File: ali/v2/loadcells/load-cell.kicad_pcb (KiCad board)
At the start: 4 copper layers, 85 x 76 mm, 108 parts, among them J1 Conn_02x01, J10 Conn_01x04, J11 Conn_01x04, J12 Conn_01x04, J2 Conn_01x05, J26 Vertical Ethernet, J3 USB_C_Receptacle_USB2.0_16P, J4 Conn_01x15, J5 Conn_02x09_Counter_Clockwise, J6 Screw_Terminal_01x02, J8 Conn_01x03, J9 Conn_01x04, SW1 SKRPANE010, U1 STM32H563RIV6, U2 AP2112K-3.3, U4 TJA1462ATK, U6 ADS124S08, U7 LAN8742AI, Y1 25 MHz, Y2 25 MHz

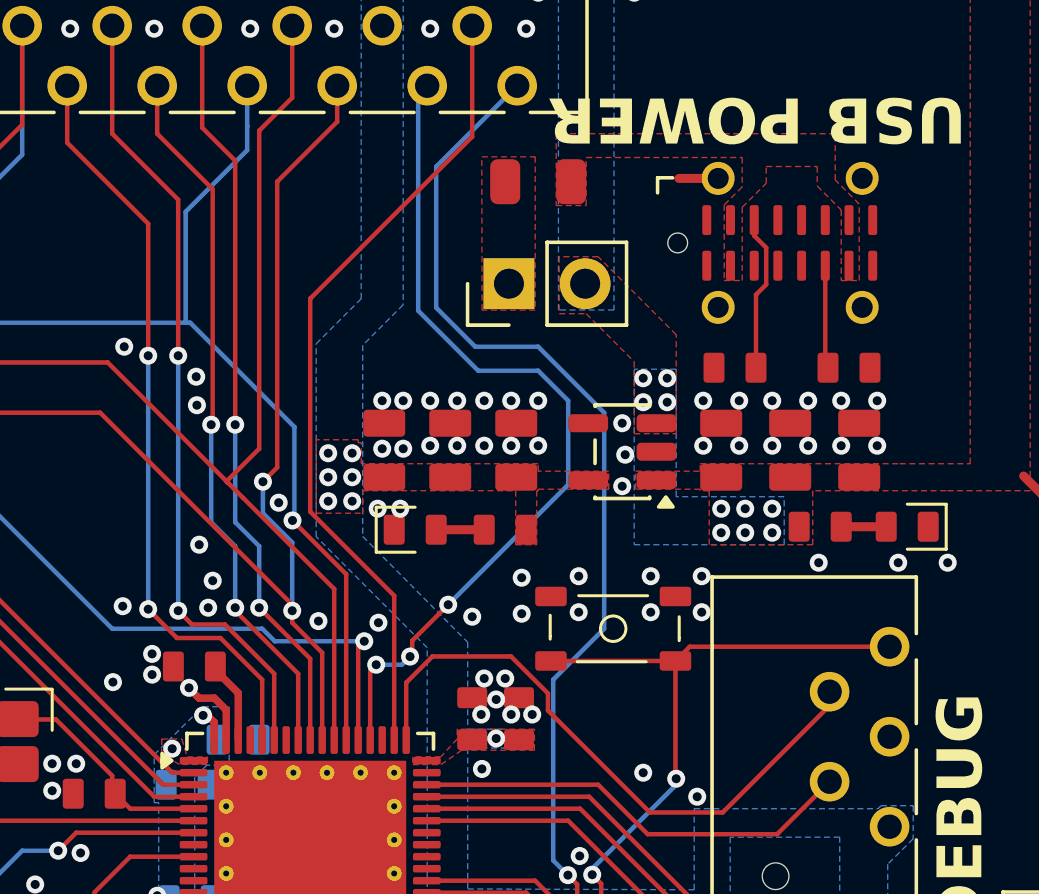
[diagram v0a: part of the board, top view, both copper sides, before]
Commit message: more clearance
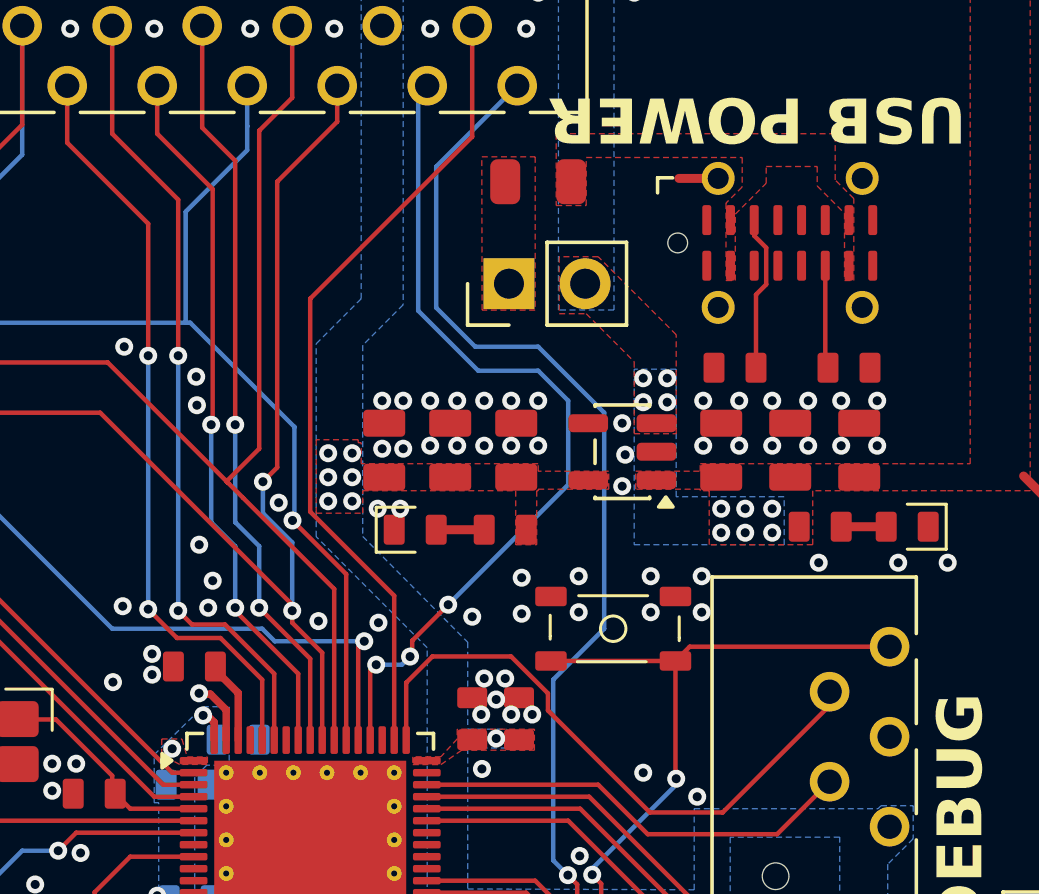
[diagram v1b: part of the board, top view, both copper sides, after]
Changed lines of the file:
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@@
 	)
 	(segment
-		(start 141.6725 93.305)
-		(end 142.0075 93.64)
+		(start 142.006912 93.477355)
+		(end 142.037312 93.507755)
 		(width 0.25)
 		(layer "F.Cu")
@@
 	)
 	(segment
-		(start 142.520673 93.64)
-		(end 142.9125 94.031827)
-		(width 0.25)
+		(start 169.699099 105.425)
+		(end 171.0125 105.425)
+		(width 0.3)
 		(layer "F.Cu")
 		(net "GND")
 	)
 	(segment
-		(start 169.699099 105.425)
-		(end 171.0125 105.425)
-		(width 0.3)
+		(start 142.037312 93.507755)
+		(end 142.388428 93.507755)
+		(width 0.25)
 		(layer "F.Cu")
 		(net "GND")
@@
 	)
 	(segment
-		(start 159.3125 76.315)
-		(end 158.0025 76.315)
-		(width 0.3)
+		(start 142.388428 93.507755)
+		(end 142.9125 94.031827)
+		(width 0.25)
 		(layer "F.Cu")
 		(net "GND")
 	)
 	(segment
-		(start 142.9125 94.031827)
-		(end 142.9125 95.0375)
-		(width 0.25)
+		(start 159.3125 76.315)
+		(end 158.0025 76.315)
+		(width 0.3)
 		(layer "F.Cu")
 		(net "GND")
@@
 	)
 	(segment
-		(start 142.0075 93.64)
-		(end 142.520673 93.64)
-		(width 0.25)
-		(layer "F.Cu")
-		(net "GND")
-	)
-	(segment
-		(start 141.6725 93.295)
-		(end 141.6725 93.305)
+		(start 142.9125 94.031827)
+		(end 142.9125 95.0375)
 		(width 0.25)
 		(layer "F.Cu")
@@
 	)
 	(via
-		(at 141.6725 93.295)
+		(at 142.006912 93.477355)
 		(size 0.6)
 		(drill 0.3)
@@
 		)
 		(min_thickness 0.15)
-		(fill yes
+		(fill
 			(thermal_gap 0.5)
 			(thermal_bridge_width 0.5)
@@
 		(polygon
 			(pts
-				(xy 160.1125 79.718008) (xy 160.1125 77.276588) (xy 160.9125 76.476588) (xy 160.9125 75.918008)
-				(xy 162.6125 75.918008) (xy 162.6125 76.568008) (xy 163.4125 77.368008) (xy 163.4125 79.718008)
-				(xy 164.0125 79.718008) (xy 164.0125 77.168008) (xy 163.2125 76.368008) (xy 163.2125 74.825) (xy 153.9125 74.825)
+				(xy 159.8825 79.718008) (xy 159.8825 77.506588) (xy 160.9125 76.476588) (xy 160.9125 75.918008)
+				(xy 162.6125 75.918008) (xy 162.6125 76.568008) (xy 163.5225 77.478008) (xy 163.5225 79.718008)
+				(xy 163.8325 79.718008) (xy 163.8325 76.988008) (xy 163.2125 76.368008) (xy 163.2125 74.825) (xy 153.9125 74.825)
 				(xy 153.9125 77.218008) (xy 154.9125 77.218008) (xy 154.9125 75.618008) (xy 160.1125 75.618008)
-				(xy 160.112182 76.598716) (xy 159.5125 77.198009) (xy 159.5125 79.718008)
+				(xy 160.112182 76.598716) (xy 159.5725 77.138048) (xy 159.5725 79.718008)
 			)
 		)
